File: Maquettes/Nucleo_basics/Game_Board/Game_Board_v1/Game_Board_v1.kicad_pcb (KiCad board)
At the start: 2 copper layers, 150 x 100 mm, 42 parts, among them CON1 MikroE-nRF-S-module, J1 TFT-RB1.8, J2 JOYSTICK, J3 AnalogIn, J4 AnalogChoice, SW1 SW_Push, SW2 SW_Push, SW3 SW_Push, SW4 SW_Push, U1 NUCLEO-L432KC, U2 4071, U3 MCP23008-xP

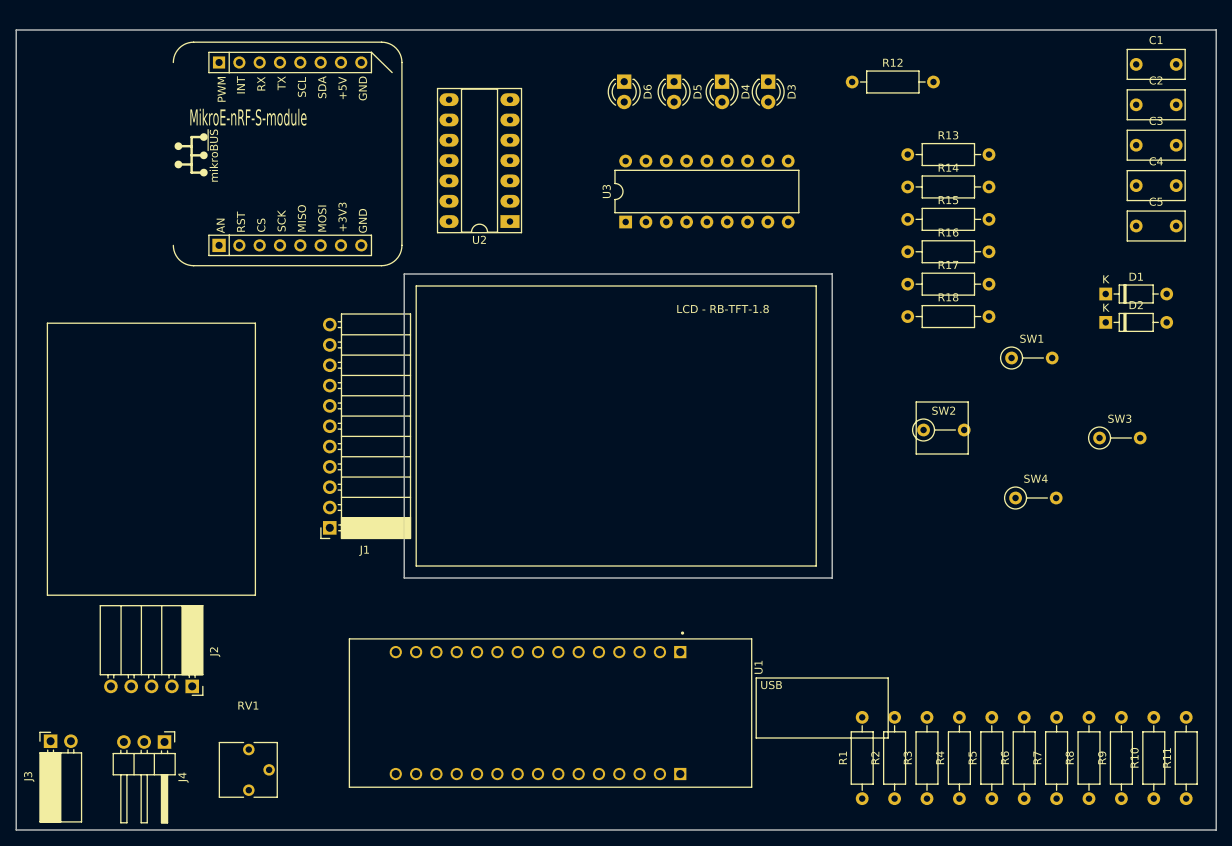
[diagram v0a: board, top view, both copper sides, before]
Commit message: Update GameBoard
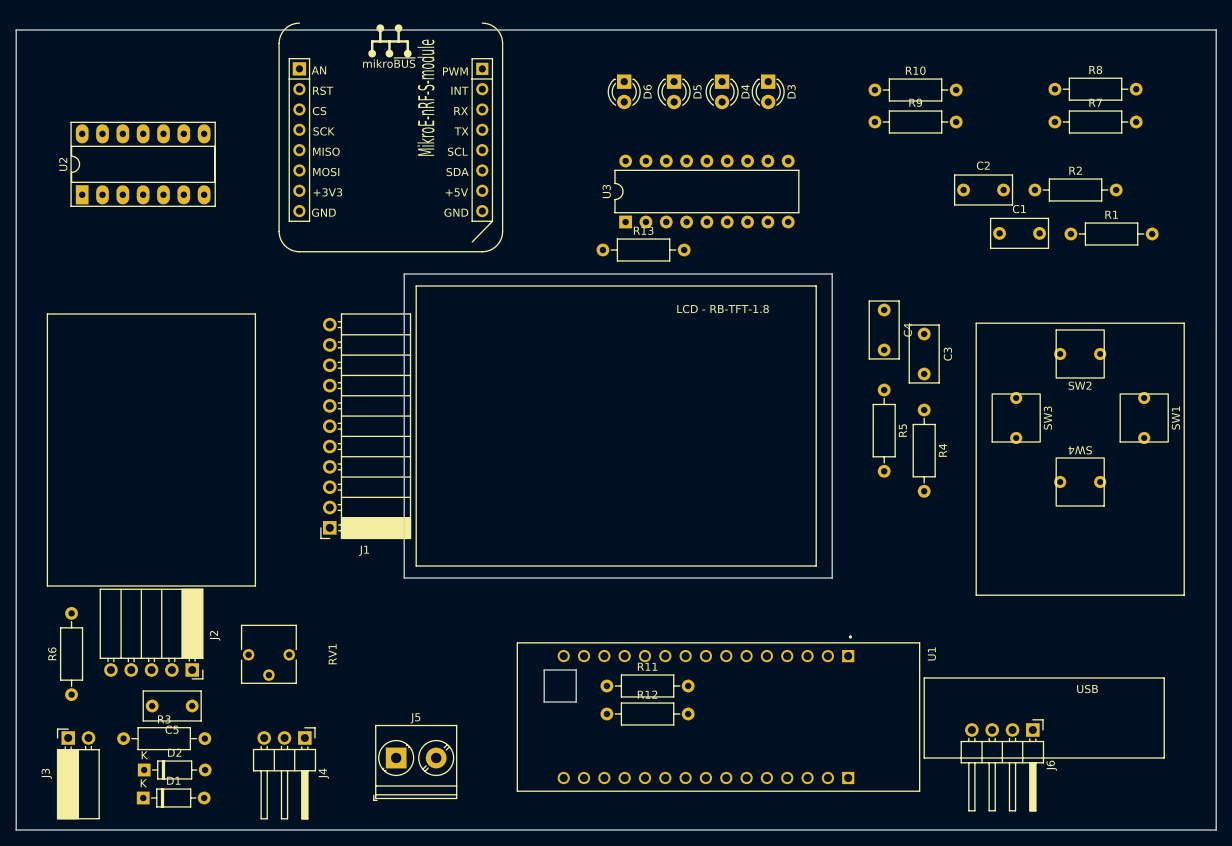
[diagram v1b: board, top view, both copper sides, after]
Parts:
- removed R14, R15: 220, Resistor_THT:R_Axial_DIN0207_L6.3mm_D2.5mm_P10.16mm_Horizontal
- removed R16, R17, R18: 1k, Resistor_THT:R_Axial_DIN0207_L6.3mm_D2.5mm_P10.16mm_Horizontal
- added J5: Conn_01x02, TerminalBlock_Phoenix:TerminalBlock_Phoenix_PT-1,5-2-5.0-H_1x02_P5.00mm_Horizontal, F.Cu at (179.5, 154.5)
- added J6: Conn_01x04, Connector_PinHeader_2.54mm:PinHeader_1x04_P2.54mm_Horizontal, F.Cu at (259.1, 151.0)
- R11, R12, R13: value 220 -> 1k
- R3: value 220 -> 1.2k
- R4: value 220 -> 12k
- R5: value 1.2k -> 12k
- R8, R9: value 12k -> 220
- RV1: value R_POT_TRIM -> R_10k
- SW1, SW2, SW3, SW4: footprint Resistor_THT:R_Axial_DIN0207_L6.3mm_D2.5mm_P5.08mm_Vertical -> LEnsE_devices:Switch
- moved D1 135.8 mm to (147.9, 159.5)
- moved D2 132.6 mm to (148.0, 156.0)
- moved C5 132.4 mm to (154.0, 148.0), turned to 180 degrees
- moved R6 119.8 mm to (138.9, 146.6)
- moved R3 100.7 mm to (145.4, 152.1), turned to 0 degrees
- moved R10 95.2 mm to (239.3, 71.0), turned to 0 degrees
- moved R9 90.0 mm to (239.3, 75.0), turned to 0 degrees
- moved R8 88.8 mm to (261.8, 70.9), turned to 0 degrees
- moved R12 84.7 mm to (205.8, 149.0)
- moved R7 84.6 mm to (261.8, 75.0), turned to 0 degrees
- moved R2 78.1 mm to (259.3, 83.5), turned to 0 degrees
- moved R1 75.2 mm to (263.8, 89.0), turned to 0 degrees
- moved R11 73.8 mm to (205.8, 145.5), turned to 0 degrees
- moved U2 53.6 mm to (140.2, 84.1), turned to 90 degrees
- moved R5 52.8 mm to (240.5, 108.5), turned to -90 degrees
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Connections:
- C1 pad 1: SW1 -> 3.3V
- C1 pad 2: GND -> SW1
- C2 pad 1: SW2 -> 3.3V
- C2 pad 2: GND -> SW2
- C3 pad 1: SW_JOY_OUT -> 3.3V
- C3 pad 2: GND -> SW3
- C4 pad 1: SW3 -> 3.3V
- C4 pad 2: GND -> SW4
- C5 pad 1: SW4 -> 3.3V
- C5 pad 2: GND -> JOYSW
- D1 pad 2: Net-(D1-A) -> AN_IN
- D2 pad 1: Net-(D1-A) -> AN_IN
- D5 pad 1: unconnected-(D5-K-Pad1) -> Net-(D5-K)
- R1 pad 1: Net-(R1-Pad1) -> SW1
- R10 pad 1: Net-(R10-Pad1) -> Net-(D6-K)
- R10 pad 2: SW3 -> GND
- R11 pad 1: Net-(R11-Pad1) -> 3.3V
- R11 pad 2: SW4 -> SCL
- R12 pad 1: Net-(D3-K) -> 3.3V
- R12 pad 2: GND -> SDA
- R13 pad 1: Net-(D4-K) -> 3.3V
- R13 pad 2: GND -> Net-(U3-~{RESET})
- R2 pad 1: Net-(R2-Pad1) -> SW2
- R3 pad 1: Net-(R1-Pad1) -> Net-(J3-Pin_2)
- R3 pad 2: SW1 -> AN_IN
- R4 pad 1: Net-(R2-Pad1) -> SW3
- R4 pad 2: SW2 -> GND
- R5 pad 1: Net-(J3-Pin_2) -> SW4
- R5 pad 2: Net-(D1-A) -> GND
- R7 pad 1: JOYSW -> Net-(D3-K)
- R7 pad 2: SW_JOY_OUT -> GND
- R8 pad 1: Net-(R10-Pad1) -> Net-(D4-K)
- R9 pad 1: Net-(R11-Pad1) -> Net-(D5-K)
- SW1 pad 2: Net-(R1-Pad1) -> SW1
- SW2 pad 2: Net-(R2-Pad1) -> SW2
- SW3 pad 2: Net-(R10-Pad1) -> SW3
- SW4 pad 2: Net-(R11-Pad1) -> SW4
- U1 pad CN3_5: SW_JOY_OUT -> JOYSW
- U1 pad CN3_7: unconnected-(U1A-PB7-PadCN3_7) -> SDA
- U1 pad CN3_8: LCD_DC -> SCL
- U1 pad CN3_9: unconnected-(U1A-PB1-PadCN3_9) -> LCD_DC
- U1 pad CN4_1: unconnected-(U1B-VIN-PadCN4_1) -> Vin
- U1 pad CN4_4: unconnected-(U1B-+5V-PadCN4_4) -> 5V
- U1 pad CN4_7: SCL -> unconnected-(U1B-PA6-PadCN4_7)
- U1 pad CN4_8: SDA -> unconnected-(U1B-PA5-PadCN4_8)
- U2 pad 1: nRF_INT -> (no net)
- U2 pad 10: (no net) -> EX_nRF_INT
- U2 pad 2: EXP_INT -> (no net)
- U2 pad 3: EX_nRF_INT -> (no net)
- U2 pad 8: (no net) -> nRF_INT
- U2 pad 9: (no net) -> EXP_INT
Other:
- outline, holes or cut-outs redrawn
